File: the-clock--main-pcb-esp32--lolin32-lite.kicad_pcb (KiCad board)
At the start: 2 copper layers, 101.6 x 38.1 mm, 0 parts

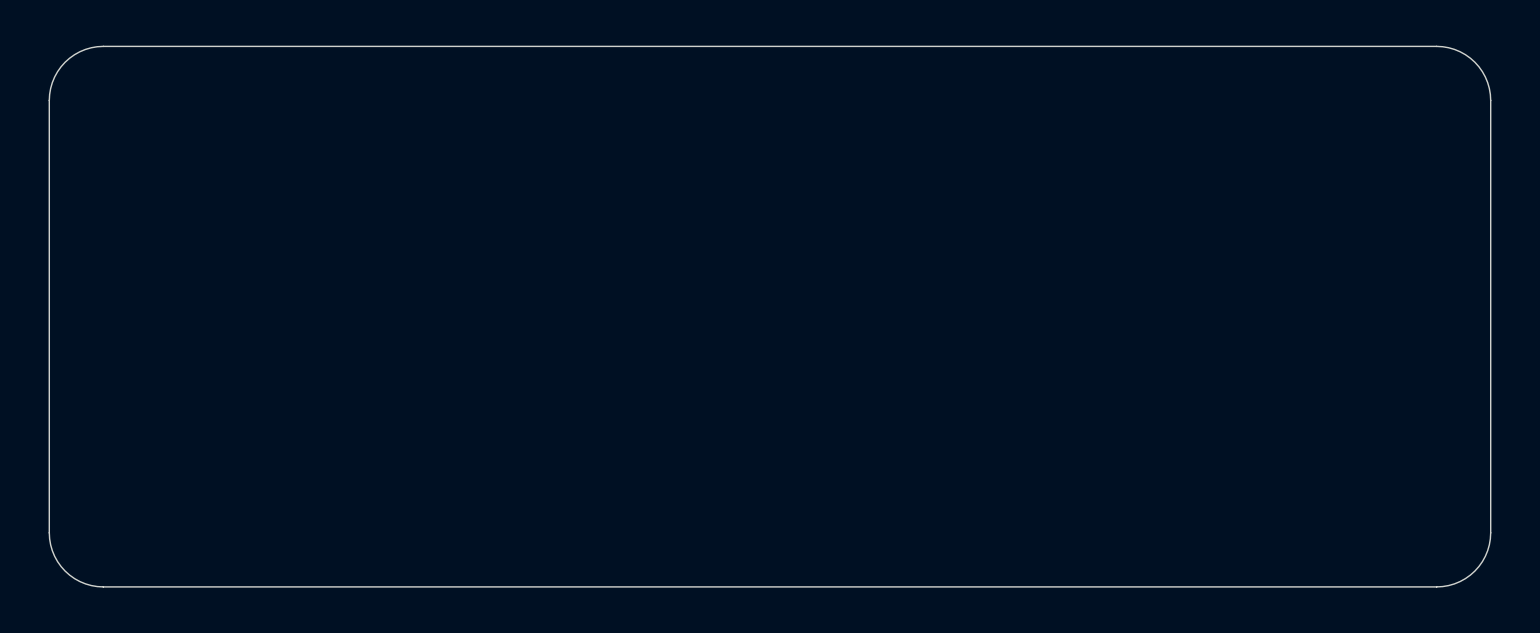
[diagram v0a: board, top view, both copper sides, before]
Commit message: pcb session 2023-11-21T22:50:08+01:00 : almost done
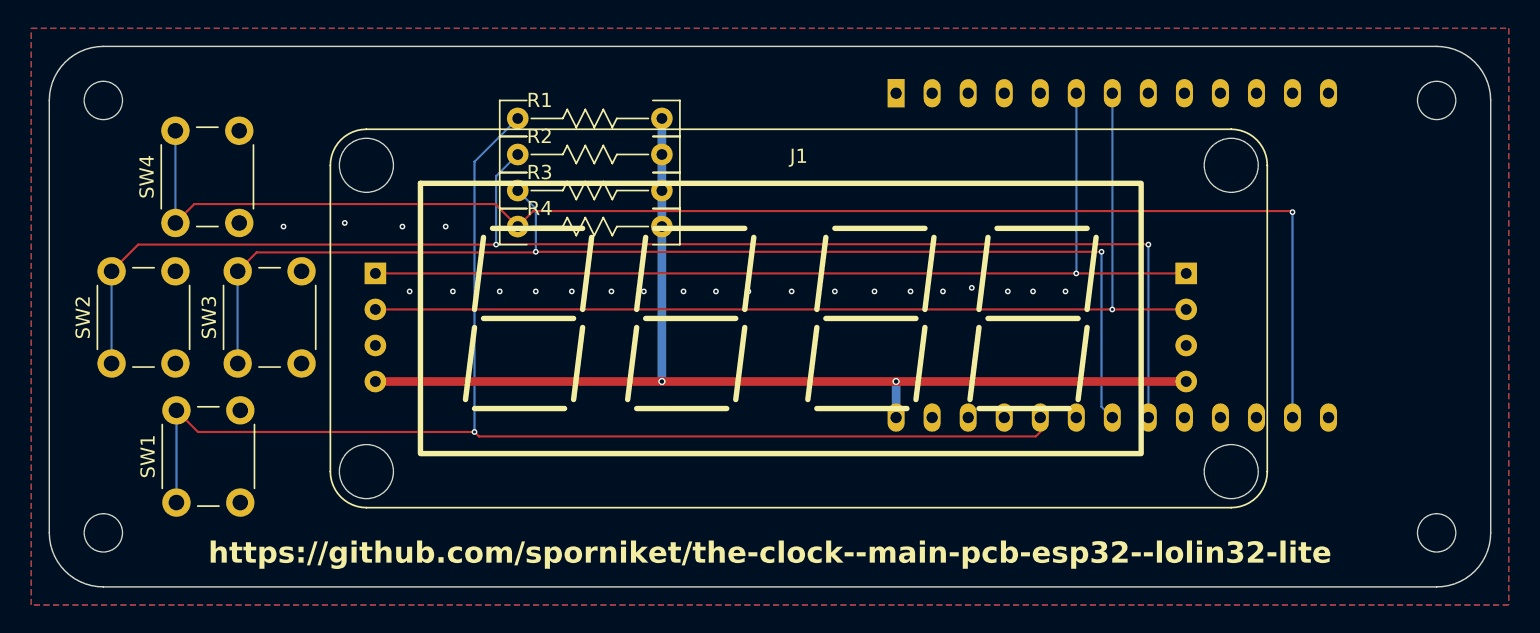
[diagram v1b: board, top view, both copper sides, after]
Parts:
- added A1: WEMOS_LOLIN32_LITE_PHY, assemblies_uc_boards:DIP-26_900_WEMOS_LOLIN32_LITE, B.Cu at (125.7, 65.5)
- added H1: M2.5, MountingHole:MountingHole_2.7mm_M2.5, F.Cu at (54.6, 54.6)
- added H2: M2.5, MountingHole:MountingHole_2.7mm_M2.5, F.Cu at (148.6, 54.6)
- added H3: M2.5, MountingHole:MountingHole_2.7mm_M2.5, F.Cu at (148.6, 85.1)
- added H4: M2.5, MountingHole:MountingHole_2.7mm_M2.5, F.Cu at (54.6, 85.1)
- added J1: Conn_01x04, assemblies_displays_modules:TM1637_7_segments_4_digits_clock_i2c, F.Cu at (103.6, 70.0)
- added R1: 5K1, commons-passives_THT:Passive_THT_resistor_W2.54mm_L10.16mm, F.Cu at (88.9, 55.9)
- added R2: 5K1, commons-passives_THT:Passive_THT_resistor_W2.54mm_L10.16mm, F.Cu at (88.9, 58.4)
- added R3: 5K1, commons-passives_THT:Passive_THT_resistor_W2.54mm_L10.16mm, F.Cu at (88.9, 61.0)
- added R4: 5K1, commons-passives_THT:Passive_THT_resistor_W2.54mm_L10.16mm, F.Cu at (88.9, 63.5)
- added SW1: SW_Push, Button_Switch_THT:SW_PUSH_6mm_H13mm, F.Cu at (59.8, 83.0)
- added SW2: SW_Push, Button_Switch_THT:SW_PUSH_6mm_H13mm, F.Cu at (55.2, 73.2)
- added SW3: SW_Push, Button_Switch_THT:SW_PUSH_6mm_H13mm, F.Cu at (64.1, 73.2)
- added SW4: SW_Push, Button_Switch_THT:SW_PUSH_6mm_H13mm, F.Cu at (59.7, 63.2)
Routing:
- net /UP/MENU: track 0.00 -> 101.4 mm, vias 0 -> 1
- net /LEFT/-: track 0.00 -> 99.6 mm, vias 0 -> 2
- net /DOWN/BACK: track 0.00 -> 92.7 mm, vias 0 -> 1
- net /RIGHT/+: track 0.00 -> 84.8 mm, vias 0 -> 2
- net VCC: track 0.00 -> 78.2 mm, vias 0 -> 2
- net /SDA: track 0.00 -> 72.4 mm, vias 0 -> 1
- net /SCL: track 0.00 -> 69.9 mm, vias 0 -> 1
- net GND: vias 0 -> 23
- added copper zone on B.Cu, net GND
- added copper zone on F.Cu, net GND
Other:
- board text added: "https://github.com/sporniket/the-clock--main-pcb-esp32--lolin32-lite"
